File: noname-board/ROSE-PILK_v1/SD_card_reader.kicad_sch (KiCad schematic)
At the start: 1 part, among them J7 Conn_02x08_Row_Letter_Last

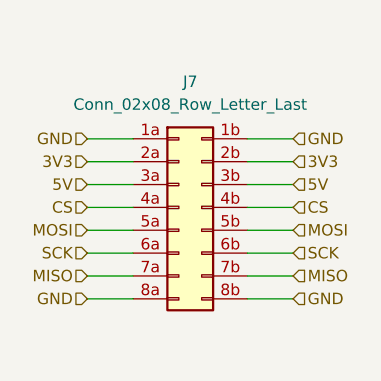
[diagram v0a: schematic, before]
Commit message: Meeting Stuff
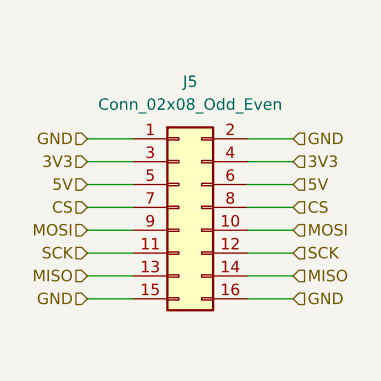
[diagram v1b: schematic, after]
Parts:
- removed J7: Conn_02x08_Row_Letter_Last, Connector_PinSocket_2.00mm:PinSocket_2x08_P2.00mm_Vertical, symbol Connector_Generic:Conn_02x08_Row_Letter_Last
- added J5: Conn_02x08_Odd_Even, Connector_PinSocket_2.00mm:PinSocket_2x08_P2.00mm_Vertical, symbol Connector_Generic:Conn_02x08_Odd_Even
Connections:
- net 3V3: now also J5.3 (Pin_3), J5.4 (Pin_4)
- net 5V: now also J5.5 (Pin_5), J5.6 (Pin_6)
- net CS: now also J5.7 (Pin_7), J5.8 (Pin_8)
- net GND: now also J5.1 (Pin_1), J5.15 (Pin_15), J5.16 (Pin_16), J5.2 (Pin_2)
- net MISO: now also J5.13 (Pin_13), J5.14 (Pin_14)
- net MOSI: now also J5.10 (Pin_10), J5.9 (Pin_9)
- net SCK: now also J5.11 (Pin_11), J5.12 (Pin_12)
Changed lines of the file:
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@@
 (kicad_sch (version 20230121) (generator eeschema)
   (paper "A4")
-  )
   (wire (pts (xy 129.54 120.65) (xy 134.62 120.65))
     (stroke (width 0) (type default))
@@
     (stroke (width 0) (type default))
   )
-  (wire (pts (xy 129.54 130.81) (xy 134.62 130.81))
+  (wire (pts (xy 129.54 118.11) (xy 134.62 118.11))
+    (stroke (width 0) (type default))
+  )
+  (wire (pts (xy 129.54 123.19) (xy 134.62 123.19))
+    (stroke (width 0) (type default))
+  )
+  (wire (pts (xy 129.54 133.35) (xy 134.62 133.35))
     (stroke (width 0) (type default))
   )
@@
     (stroke (width 0) (type default))
   )
-  (wire (pts (xy 129.54 123.19) (xy 134.62 123.19))
-    (stroke (width 0) (type default))
-  )
   (wire (pts (xy 129.54 125.73) (xy 134.62 125.73))
     (stroke (width 0) (type default))
   )
-  (wire (pts (xy 129.54 128.27) (xy 134.62 128.27))
+  (wire (pts (xy 129.54 130.81) (xy 134.62 130.81))
     (stroke (width 0) (type default))
   )
-  (wire (pts (xy 129.54 118.11) (xy 134.62 118.11))
+  (wire (pts (xy 129.54 128.27) (xy 134.62 128.27))
     (stroke (width 0) (type default))
   )
@@
   )
   (wire (pts (xy 111.76 120.65) (xy 116.84 120.65))
-    (stroke (width 0) (type default))
-  )
-  (wire (pts (xy 129.54 133.35) (xy 134.62 133.35))
     (stroke (width 0) (type default))
   )
@@
     (effects (font (size 1.27 1.27)) (justify right))
   )
-  (symbol (lib_id "Connector_Generic:Conn_02x08_Row_Letter_Last") (at 121.92 125.73 0) (unit 1)
+  (symbol (lib_id "Connector_Generic:Conn_02x08_Odd_Even") (at 121.92 125.73 0) (unit 1)
     (in_bom yes) (on_board yes) (dnp no) (fields_autoplaced)
-    (property "Reference" "J7" (at 123.19 111.76 0)
+    (property "Reference" "J5" (at 123.19 111.76 0)
       (effects (font (size 1.27 1.27)))
     )
-    (property "Value" "Conn_02x08_Row_Letter_Last" (at 123.19 114.3 0)
+    (property "Value" "Conn_02x08_Odd_Even" (at 123.19 114.3 0)
       (effects (font (size 1.27 1.27)))
     )
@@
       (effects (font (size 1.27 1.27)) hide)
     )
-    (pin "1a")
-    (pin "1b")
-    (pin "2a")
-    (pin "2b")
-    (pin "3a")
-    (pin "3b")
-    (pin "4a")
-    (pin "4b")
-    (pin "5a")
-    (pin "5b")
-    (pin "6a")
-    (pin "6b")
-    (pin "7a")
-    (pin "7b")
-    (pin "8a")
-    (pin "8b")
+    (pin "1")
+    (pin "10")
+    (pin "11")
+    (pin "12")
+    (pin "13")
+    (pin "14")
+    (pin "15")
+    (pin "16")
+    (pin "2")
+    (pin "3")
+    (pin "4")
+    (pin "5")
+    (pin "6")
+    (pin "7")
+    (pin "8")
+    (pin "9")
     (instances
       (project "ROSE-PILK_v1"
         (path "/3dfb9737-68ba-4ca9-8085-72e4f57f9e50/bba6feb6-0708-4b51-a731-0bb8ba53ae80"
-          (reference "J7") (unit 1)
+          (reference "J5") (unit 1)
         )
       )

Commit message: Schematics
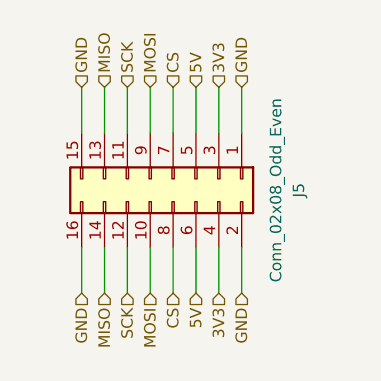
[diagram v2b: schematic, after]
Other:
- moved on the sheet: J5
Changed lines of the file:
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@@
 (kicad_sch (version 20230121) (generator eeschema)
   (paper "A4")
-  (wire (pts (xy 129.54 120.65) (xy 134.62 120.65))
+  (wire (pts (xy 126.365 130.175) (xy 126.365 135.255))
     (stroke (width 0) (type default))
   )
-  (wire (pts (xy 111.76 123.19) (xy 116.84 123.19))
+  (wire (pts (xy 123.825 112.395) (xy 123.825 117.475))
     (stroke (width 0) (type default))
   )
-  (wire (pts (xy 129.54 118.11) (xy 134.62 118.11))
+  (wire (pts (xy 128.905 130.175) (xy 128.905 135.255))
     (stroke (width 0) (type default))
   )
-  (wire (pts (xy 129.54 123.19) (xy 134.62 123.19))
+  (wire (pts (xy 123.825 130.175) (xy 123.825 135.255))
     (stroke (width 0) (type default))
   )
-  (wire (pts (xy 129.54 133.35) (xy 134.62 133.35))
+  (wire (pts (xy 113.665 130.175) (xy 113.665 135.255))
     (stroke (width 0) (type default))
   )
-  (wire (pts (xy 111.76 130.81) (xy 116.84 130.81))
+  (wire (pts (xy 116.205 112.395) (xy 116.205 117.475))
     (stroke (width 0) (type default))
   )
-  (wire (pts (xy 129.54 125.73) (xy 134.62 125.73))
+  (wire (pts (xy 121.285 130.175) (xy 121.285 135.255))
     (stroke (width 0) (type default))
   )
-  (wire (pts (xy 129.54 130.81) (xy 134.62 130.81))
+  (wire (pts (xy 116.205 130.175) (xy 116.205 135.255))
     (stroke (width 0) (type default))
   )
-  (wire (pts (xy 129.54 128.27) (xy 134.62 128.27))
+  (wire (pts (xy 118.745 130.175) (xy 118.745 135.255))
     (stroke (width 0) (type default))
   )
-  (wire (pts (xy 129.54 135.89) (xy 134.62 135.89))
+  (wire (pts (xy 111.125 130.175) (xy 111.125 135.255))
     (stroke (width 0) (type default))
   )
-  (wire (pts (xy 111.76 133.35) (xy 116.84 133.35))
+  (wire (pts (xy 113.665 112.395) (xy 113.665 117.475))
     (stroke (width 0) (type default))
   )
-  (wire (pts (xy 111.76 128.27) (xy 116.84 128.27))
+  (wire (pts (xy 118.745 112.395) (xy 118.745 117.475))
     (stroke (width 0) (type default))
   )
-  (wire (pts (xy 111.76 118.11) (xy 116.84 118.11))
+  (wire (pts (xy 128.905 112.395) (xy 128.905 117.475))
     (stroke (width 0) (type default))
   )
-  (wire (pts (xy 111.76 125.73) (xy 116.84 125.73))
+  (wire (pts (xy 121.285 112.395) (xy 121.285 117.475))
     (stroke (width 0) (type default))
   )
-  (wire (pts (xy 111.76 120.65) (xy 116.84 120.65))
+  (wire (pts (xy 126.365 112.395) (xy 126.365 117.475))
     (stroke (width 0) (type default))
   )
-  (wire (pts (xy 111.76 135.89) (xy 116.84 135.89))
+  (wire (pts (xy 111.125 112.395) (xy 111.125 117.475))
     (stroke (width 0) (type default))
   )
-  (hierarchical_label "GND" (shape input) (at 111.76 135.89 180) (fields_autoplaced)
+  (hierarchical_label "GND" (shape input) (at 111.125 112.395 90) (fields_autoplaced)
+    (effects (font (size 1.27 1.27)) (justify left))
+  )
+  (hierarchical_label "GND" (shape input) (at 111.125 135.255 270) (fields_autoplaced)
     (effects (font (size 1.27 1.27)) (justify right))
   )
-  (hierarchical_label "GND" (shape input) (at 134.62 135.89 0) (fields_autoplaced)
+  (hierarchical_label "MISO" (shape input) (at 113.665 135.255 270) (fields_autoplaced)
+    (effects (font (size 1.27 1.27)) (justify right))
+  )
+  (hierarchical_label "MOSI" (shape input) (at 118.745 135.255 270) (fields_autoplaced)
+    (effects (font (size 1.27 1.27)) (justify right))
+  )
+  (hierarchical_label "SCK" (shape input) (at 116.205 135.255 270) (fields_autoplaced)
+    (effects (font (size 1.27 1.27)) (justify right))
+  )
+  (hierarchical_label "GND" (shape input) (at 128.905 112.395 90) (fields_autoplaced)
     (effects (font (size 1.27 1.27)) (justify left))
   )
-  (hierarchical_label "MISO" (shape input) (at 134.62 133.35 0) (fields_autoplaced)
+  (hierarchical_label "SCK" (shape input) (at 116.205 112.395 90) (fields_autoplaced)
     (effects (font (size 1.27 1.27)) (justify left))
   )
-  (hierarchical_label "MOSI" (shape input) (at 134.62 128.27 0) (fields_autoplaced)
+  (hierarchical_label "MISO" (shape input) (at 113.665 112.395 90) (fields_autoplaced)
     (effects (font (size 1.27 1.27)) (justify left))
   )
-  (hierarchical_label "SCK" (shape input) (at 134.62 130.81 0) (fields_autoplaced)
+  (hierarchical_label "3V3" (shape input) (at 126.365 135.255 270) (fields_autoplaced)
+    (effects (font (size 1.27 1.27)) (justify right))
+  )
+  (hierarchical_label "3V3" (shape input) (at 126.365 112.395 90) (fields_autoplaced)
     (effects (font (size 1.27 1.27)) (justify left))
   )
-  (hierarchical_label "GND" (shape input) (at 111.76 118.11 180) (fields_autoplaced)
+  (hierarchical_label "GND" (shape input) (at 128.905 135.255 270) (fields_autoplaced)
     (effects (font (size 1.27 1.27)) (justify right))
   )
-  (hierarchical_label "SCK" (shape input) (at 111.76 130.81 180) (fields_autoplaced)
+  (hierarchical_label "CS" (shape input) (at 121.285 112.395 90) (fields_autoplaced)
+    (effects (font (size 1.27 1.27)) (justify left))
+  )
+  (hierarchical_label "5V" (shape input) (at 123.825 135.255 270) (fields_autoplaced)
     (effects (font (size 1.27 1.27)) (justify right))
   )
-  (hierarchical_label "MISO" (shape input) (at 111.76 133.35 180) (fields_autoplaced)
+  (hierarchical_label "5V" (shape input) (at 123.825 112.395 90) (fields_autoplaced)
+    (effects (font (size 1.27 1.27)) (justify left))
+  )
+  (hierarchical_label "CS" (shape input) (at 121.285 135.255 270) (fields_autoplaced)
     (effects (font (size 1.27 1.27)) (justify right))
   )
-  (hierarchical_label "3V3" (shape input) (at 134.62 120.65 0) (fields_autoplaced)
+  (hierarchical_label "MOSI" (shape input) (at 118.745 112.395 90) (fields_autoplaced)
     (effects (font (size 1.27 1.27)) (justify left))
   )
-  (hierarchical_label "3V3" (shape input) (at 111.76 120.65 180) (fields_autoplaced)
-    (effects (font (size 1.27 1.27)) (justify right))
-  )
-  (hierarchical_label "GND" (shape input) (at 134.62 118.11 0) (fields_autoplaced)
-    (effects (font (size 1.27 1.27)) (justify left))
-  )
-  (hierarchical_label "CS" (shape input) (at 111.76 125.73 180) (fields_autoplaced)
-    (effects (font (size 1.27 1.27)) (justify right))
-  )
-  (hierarchical_label "5V" (shape input) (at 134.62 123.19 0) (fields_autoplaced)
-    (effects (font (size 1.27 1.27)) (justify left))
-  )
-  (hierarchical_label "5V" (shape input) (at 111.76 123.19 180) (fields_autoplaced)
-    (effects (font (size 1.27 1.27)) (justify right))
-  )
-  (hierarchical_label "CS" (shape input) (at 134.62 125.73 0) (fields_autoplaced)
-    (effects (font (size 1.27 1.27)) (justify left))
-  )
-  (hierarchical_label "MOSI" (shape input) (at 111.76 128.27 180) (fields_autoplaced)
-    (effects (font (size 1.27 1.27)) (justify right))
-  )
-  (symbol (lib_id "Connector_Generic:Conn_02x08_Odd_Even") (at 121.92 125.73 0) (unit 1)
+  (symbol (lib_id "Connector_Generic:Conn_02x08_Odd_Even") (at 121.285 122.555 270) (unit 1)
     (in_bom yes) (on_board yes) (dnp no) (fields_autoplaced)
-    (property "Reference" "J5" (at 123.19 111.76 0)
+    (property "Reference" "J5" (at 135.255 123.825 0)
       (effects (font (size 1.27 1.27)))
     )
-    (property "Value" "Conn_02x08_Odd_Even" (at 123.19 114.3 0)
+    (property "Value" "Conn_02x08_Odd_Even" (at 132.715 123.825 0)
       (effects (font (size 1.27 1.27)))
     )
-    (property "Footprint" "Connector_PinSocket_2.00mm:PinSocket_2x08_P2.00mm_Vertical" (at 121.92 125.73 0)
+    (property "Footprint" "Connector_PinSocket_2.00mm:PinSocket_2x08_P2.00mm_Vertical" (at 121.285 122.555 0)
       (effects (font (size 1.27 1.27)) hide)
     )
-    (property "Datasheet" "~" (at 121.92 125.73 0)
+    (property "Datasheet" "~" (at 121.285 122.555 0)
       (effects (font (size 1.27 1.27)) hide)
     )
